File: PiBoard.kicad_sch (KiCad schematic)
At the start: 0 parts

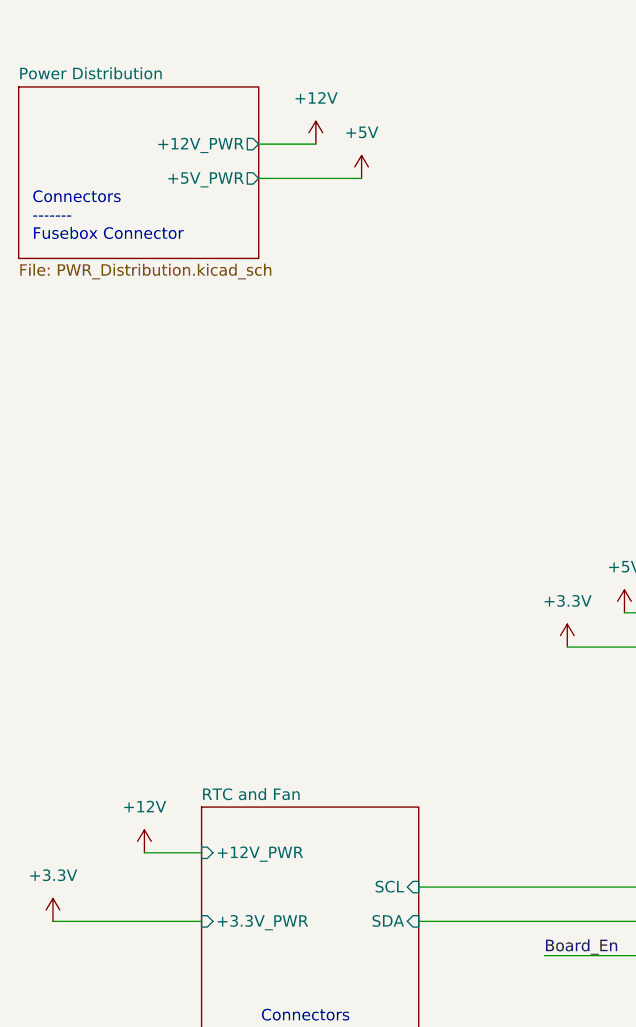
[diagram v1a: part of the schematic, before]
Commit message: moved some stuff around
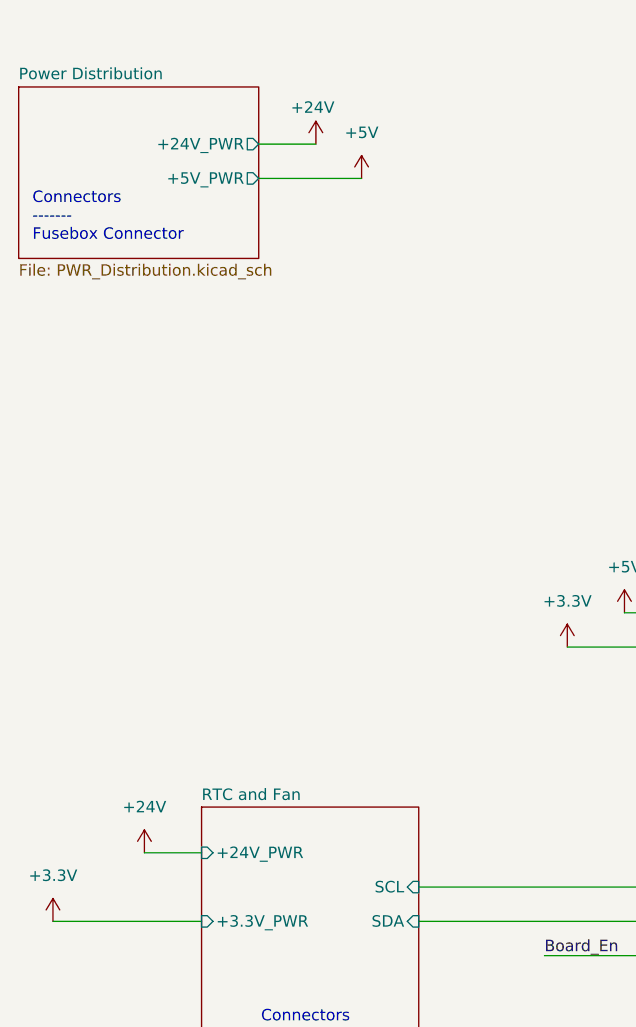
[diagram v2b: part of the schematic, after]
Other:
- sheet Power Distribution ports: added +24V_PWR; removed +12V_PWR
- sheet RTC and Fan ports: added +24V_PWR; removed +12V_PWR
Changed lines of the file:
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@@
 		(on_board yes)
 		(dnp no)
-		(fields_autoplaced yes)
 		(property "Reference" "#PWR066"
 			(at 77.47 48.26 0)
@@
 			)
 		)
-		(property "Value" "+12V"
-			(at 77.47 39.37 0)
-			(effects
-				(font
-					(size 1.27 1.27)
-				)
+		(property "Value" "+24V"
+			(at 74.676 40.386 0)
+			(effects
+				(font
+					(size 1.27 1.27)
+				)
+				(justify left)
 			)
 		)
@@
 			)
 		)
-		(property "Value" "+12V"
+		(property "Value" "+24V"
 			(at 58.42 118.11 0)
 			(effects
@@
 			)
 		)
-		(pin "+12V_PWR" output
+		(pin "+24V_PWR" output
 			(at 71.12 44.45 0)
 			(effects
@@
 			)
 		)
-		(pin "+12V_PWR" input
+		(pin "+24V_PWR" input
 			(at 64.77 123.19 180)
 			(effects
